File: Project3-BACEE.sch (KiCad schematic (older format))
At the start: 13 parts, among them U1 24LC1025, U2 24LC1025, U3 DS1337_CSP, U4 ATMEGA328P-AU, Y1 Crystal 32MHz, Y2 Crystal 16MHz

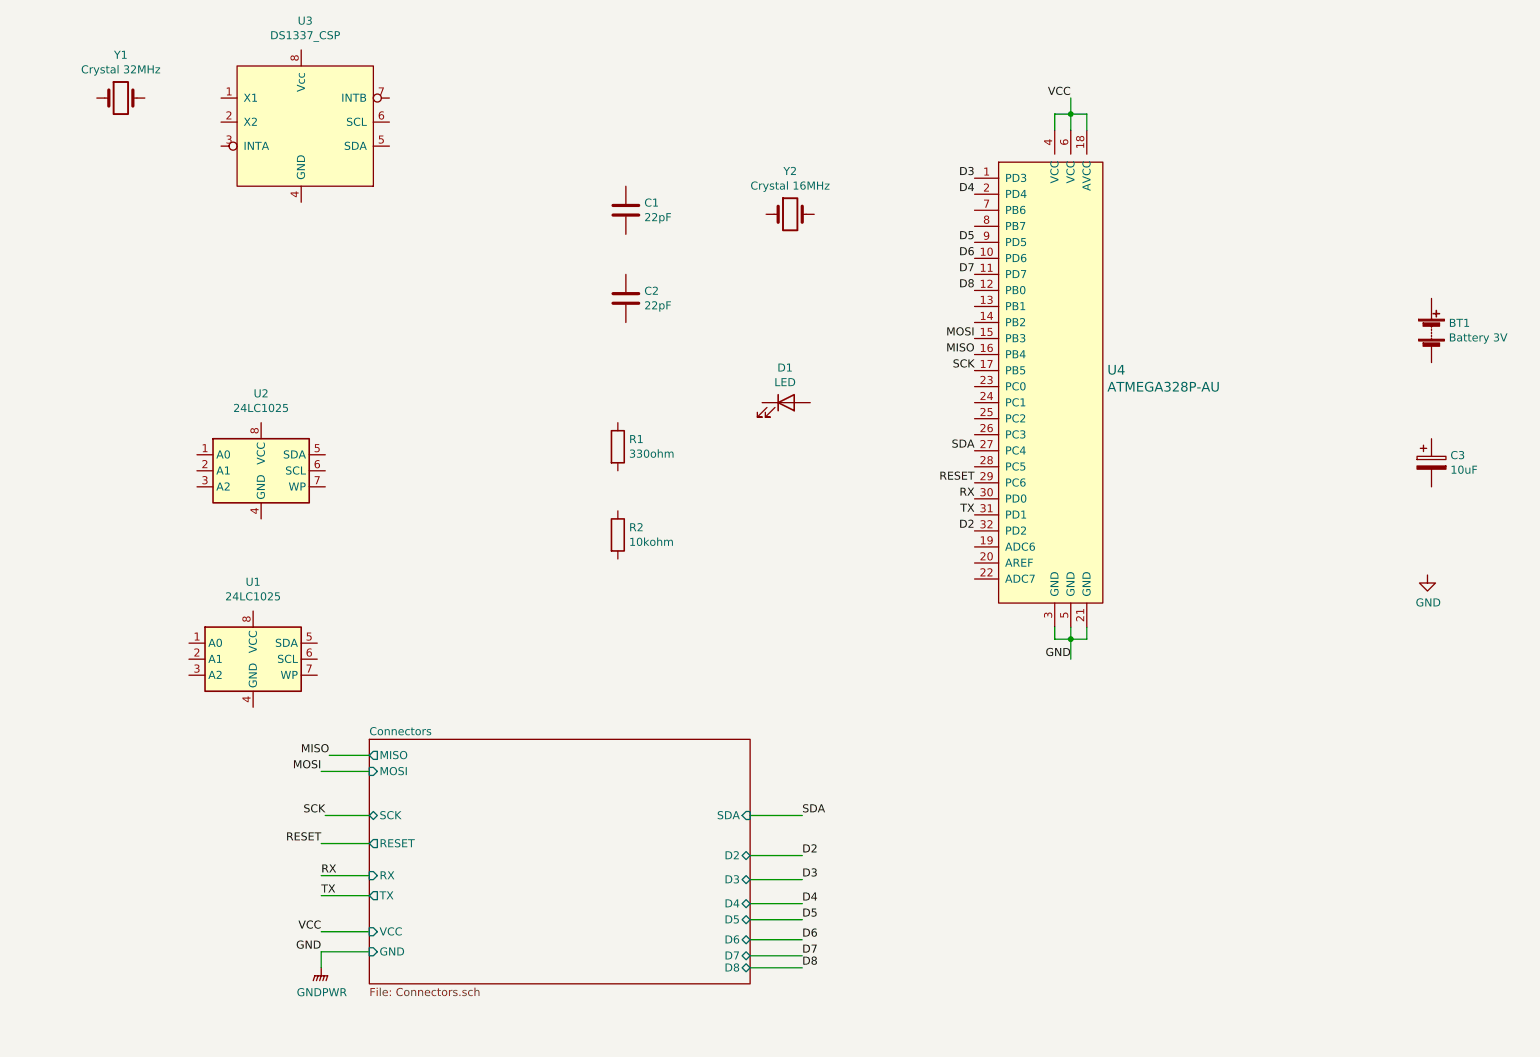
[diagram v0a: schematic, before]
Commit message: added comments
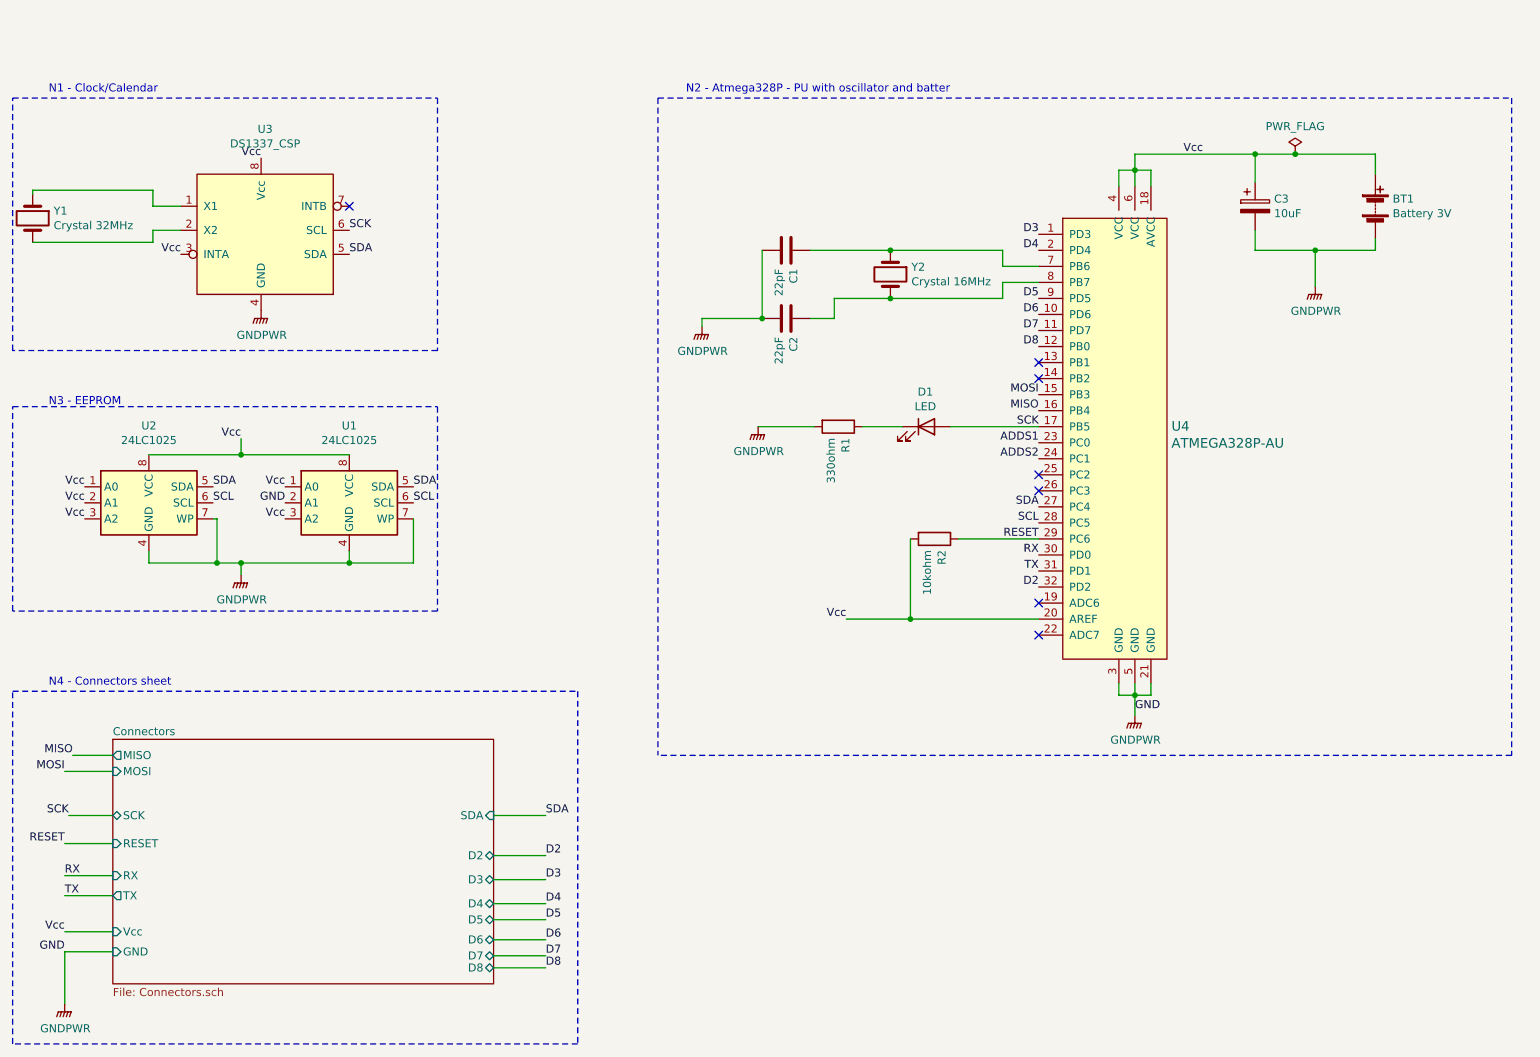
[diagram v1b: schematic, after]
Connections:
- net GND is gone; now on net GNDPWR: U4.21 (GND), U4.3 (GND), U4.5 (GND)
- net VCC is gone; now on net Vcc: U4.18 (AVCC), U4.4 (VCC), U4.6 (VCC)
- net RESET: now also R2.1
- net SCK: now also D1.2 (A), U3.6 (SCL)
- net SDA: now also U1.5 (SDA), U2.5 (SDA), U3.5 (SDA)
- net Vcc: now reaches BT1.1 (+)
- net Vcc: now also C3.1, R2.2, U1.1 (A0), U1.3 (A2), U1.8 (VCC), U2.1 (A0), U2.2 (A1), U2.3 (A2), U2.8 (VCC), U3.3 (INTA), U3.8 (Vcc), U4.20 (AREF)
- net GNDPWR: now reaches BT1.2 (-)
- net GNDPWR: now also C1.2, C2.2, C3.2, R1.2, U1.2 (A1), U1.4 (GND), U1.7 (WP), U2.4 (GND), U2.7 (WP), U3.4 (GND)
- net at C1.1: now also U4.7 (PB6), Y2.1
- net at C2.1: now also U4.8 (PB7), Y2.2
- net at D1.1 (K): now also R1.1
- net SCL: now reaches U2.6 (SCL)
- net SCL: now also U1.6 (SCL), U4.28 (PC5)
- net ADDS1: now reaches U4.23 (PC0)
- net ADDS2: now reaches U4.24 (PC1)
- net at U3.1 (X1): now also Y1.1
- net at U3.2 (X2): now also Y1.2
- no-connect marks 0 -> 7
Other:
- note added: "N1 - Clock/Calendar"
- note added: "N2 - Atmega328P - PU with oscillator and batter"
- note added: "N3 - EEPROM"
- note added: "N4 - Connectors sheet"
- moved on the sheet: BT1, C1, C2, C3, D1, R1, R2, U1, U2, U3, U4, Y1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
